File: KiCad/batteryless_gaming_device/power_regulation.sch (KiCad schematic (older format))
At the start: 16 parts, among them U500 TPS61201DRC

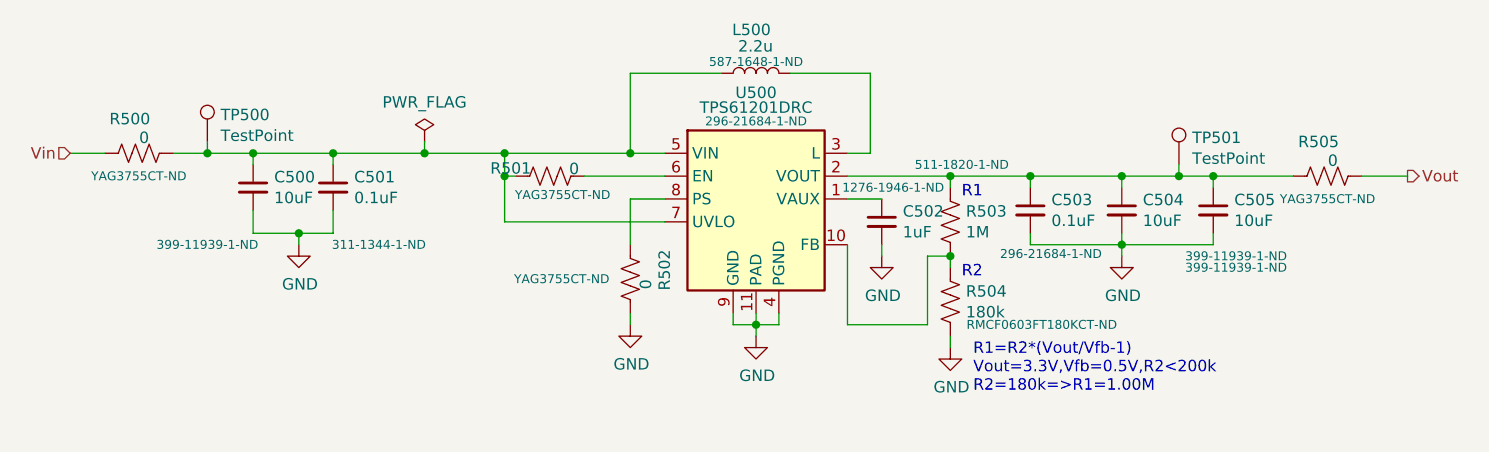
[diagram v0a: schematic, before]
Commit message: oh ya
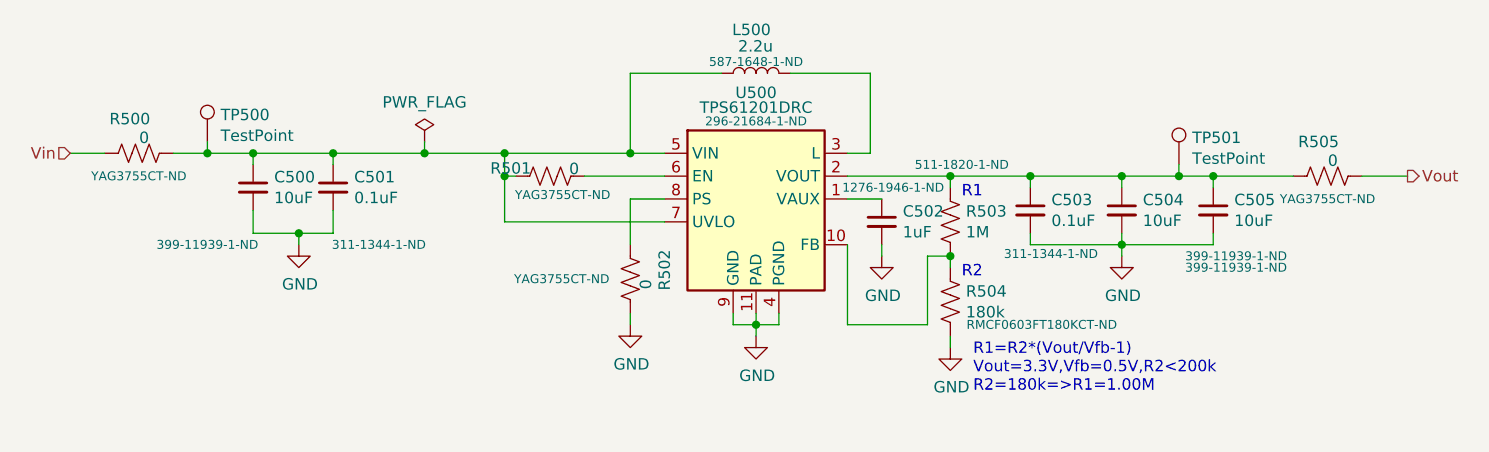
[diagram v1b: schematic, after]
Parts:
- C503: Digikey PN 296-21684-1-ND -> 311-1344-1-ND
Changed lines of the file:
@@
 F 2 "Capacitor_SMD:C_0603_1608Metric_Pad1.08x0.95mm_HandSolder" H 6500 4000 50  0001 C CNN
 F 3 "~" H 6500 4000 50  0001 C CNN
-F 4 "296-21684-1-ND" H 6590 3810 39  0000 C CNN "Digikey PN"
+F 4 "311-1344-1-ND" H 6590 3810 39  0000 C CNN "Digikey PN"
 	1    6500 4000
 	1    0    0    -1

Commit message: updated
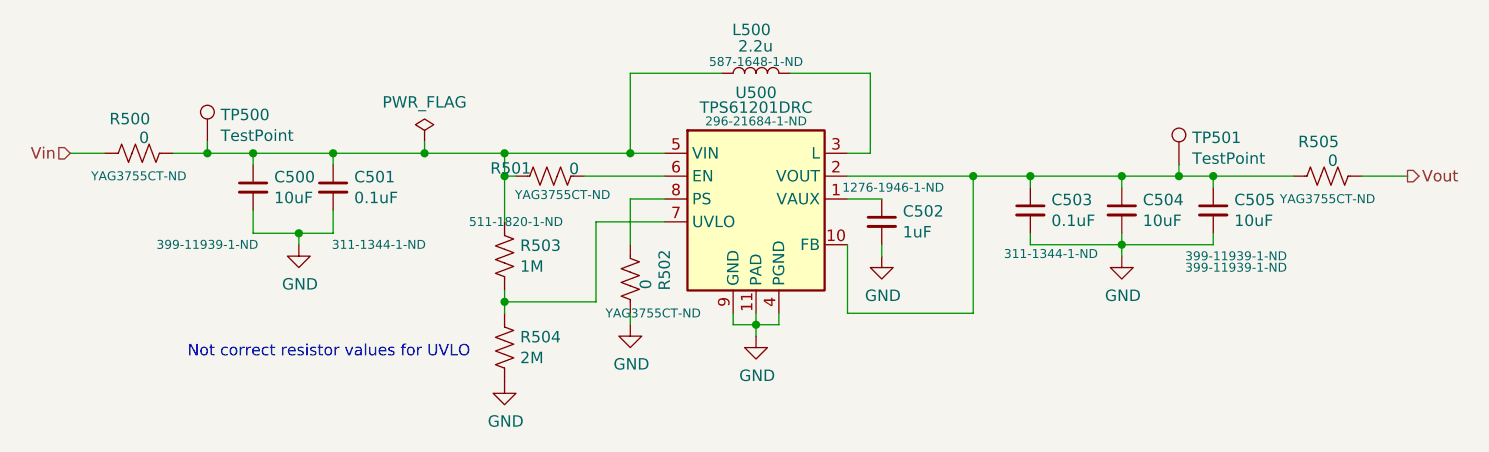
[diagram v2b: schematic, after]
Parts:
- R504: value 180k -> 2M; Digikey PN RMCF0603FT180KCT-ND -> (none)
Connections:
- net at R503.2, R504.1: now also U500.7 (UVLO); no longer U500.10 (FB)
- net at C503.1, C504.1, C505.1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: now also U500.10 (FB); no longer R503.1
- net at C500.1, C501.1, L500.1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: now also R503.1; no longer U500.7 (UVLO)
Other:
- note added: "Not correct resistor values for UVLO"
- note removed: "R1"
- note removed: "R1=R2*(Vout/Vfb-1)\nVout=3.3V,Vfb=0.5V,R2<200k\nR2=180k=>R1=1.00M"
- note removed: "R2"
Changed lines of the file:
@@
-	1    0    0    -1
-$EndComp
-$Comp
-L Device:R_US R?
-U 1 1 61950619
-P 6150 4050
-AR Path="/61950619" Ref="R?"  Part="1"
-AR Path="/61941831/61950619" Ref="R503"  Part="1"
-F 0 "R503" H 6218 4096 50  0000 L CNN
-F 1 "1M" H 6218 4005 50  0000 L CNN
-F 2 "Resistor_SMD:R_0603_1608Metric_Pad0.98x0.95mm_HandSolder" V 6190 4040 50  0001 C CNN
-F 3 "~" H 6150 4050 50  0001 C CNN
-F 4 "511-1820-1-ND" H 6200 4300 39  0000 C CNN "Digikey PN"
-	1    6150 4050
-	1    0    0    -1
-$EndComp
-$Comp
-L Device:R_US R?
-U 1 1 6195061F
-P 6150 4400
-AR Path="/6195061F" Ref="R?"  Part="1"
-AR Path="/61941831/6195061F" Ref="R504"  Part="1"
-F 0 "R504" H 6218 4446 50  0000 L CNN
-F 1 "180k" H 6218 4355 50  0000 L CNN
-F 2 "Resistor_SMD:R_0603_1608Metric_Pad0.98x0.95mm_HandSolder" V 6190 4390 50  0001 C CNN
-F 3 "~" H 6150 4400 50  0001 C CNN
-F 4 "RMCF0603FT180KCT-ND" H 6550 4300 39  0000 C CNN "Digikey PN"
-	1    6150 4400
 	1    0    0    -1
 $EndComp
@@
 	1    0    0    -1
 $EndComp
-Wire Wire Line
-	5700 3850 6150 3850
-Wire Wire Line
-	6150 3900 6150 3850
-Connection ~ 6150 3850
-Wire Wire Line
-	6150 3850 6500 3850
-Wire Wire Line
-	6150 4200 6150 4250
-$Comp
-L power:GND #PWR?
-U 1 1 61950666
-P 6150 4600
-AR Path="/61950666" Ref="#PWR?"  Part="1"
-AR Path="/61941831/61950666" Ref="#PWR0504"  Part="1"
-F 0 "#PWR0504" H 6150 4350 50  0001 C CNN
-F 1 "GND" H 6155 4427 50  0000 C CNN
-F 2 "" H 6150 4600 50  0001 C CNN
-F 3 "" H 6150 4600 50  0001 C CNN
-	1    6150 4600
-	1    0    0    -1
-$EndComp
-Wire Wire Line
-	6150 4600 6150 4550
-Wire Wire Line
-	6150 4200 6050 4200
-Wire Wire Line
-	6050 4200 6050 4500
-Wire Wire Line
-	6050 4500 5700 4500
-Wire Wire Line
-	5700 4500 5700 4150
-Connection ~ 6150 4200
-Text Notes 6250 4800 0    50   ~ 0
-R1=R2*(Vout/Vfb-1)\nVout=3.3V,Vfb=0.5V,R2<200k\nR2=180k=>R1=1.00M
-Text Notes 6200 3950 0    50   ~ 0
-R1
-Text Notes 6200 4300 0    50   ~ 0
-R2
 Wire Wire Line
 	2300 3750 2450 3750
@@
 F 2 "Resistor_SMD:R_0805_2012Metric_Pad1.20x1.40mm_HandSolder" V 4790 4290 50  0001 C CNN
 F 3 "~" H 4750 4300 50  0001 C CNN
-F 4 "YAG3755CT-ND" H 4450 4300 39  0000 C CNN "Digikey PN"
+F 4 "YAG3755CT-ND" H 4850 4150 39  0000 C CNN "Digikey PN"
 	1    4750 4300
 	1    0    0    -1
@@
 	4200 3850 4250 3850
 Wire Wire Line
-	4200 4050 4900 4050
-Wire Wire Line
 	4200 3850 4200 3750
 Connection ~ 4200 3850
@@
 Wire Wire Line
 	3850 3750 4200 3750
+$Comp
+L Device:R_US R?
+U 1 1 61B125C6
+P 4200 4200
+AR Path="/61B125C6" Ref="R?"  Part="1"
+AR Path="/61941831/61B125C6" Ref="R503"  Part="1"
+F 0 "R503" H 4268 4246 50  0000 L CNN
+F 1 "1M" H 4268 4155 50  0000 L CNN
+F 2 "Resistor_SMD:R_0603_1608Metric_Pad0.98x0.95mm_HandSolder" V 4240 4190 50  0001 C CNN
+F 3 "~" H 4200 4200 50  0001 C CNN
+F 4 "511-1820-1-ND" H 4250 4350 39  0000 C CNN "Digikey PN"
+	1    4200 4200
+	1    0    0    -1
+$EndComp
+Wire Wire Line
+	5700 3850 6250 3850
+$Comp
+L Device:R_US R?
+U 1 1 61B1718F
+P 4200 4600
+AR Path="/61B1718F" Ref="R?"  Part="1"
+AR Path="/61941831/61B1718F" Ref="R504"  Part="1"
+F 0 "R504" H 4268 4646 50  0000 L CNN
+F 1 "2M" H 4268 4555 50  0000 L CNN
+F 2 "Resistor_SMD:R_0603_1608Metric_Pad0.98x0.95mm_HandSolder" V 4240 4590 50  0001 C CNN
+F 3 "~" H 4200 4600 50  0001 C CNN
+F 4 "" H 3950 4750 39  0000 C CNN "Digikey PN"
+	1    4200 4600
+	1    0    0    -1
+$EndComp
+$Comp
+L power:GND #PWR?
+U 1 1 61B17DBB
+P 4200 4750
+AR Path="/61B17DBB" Ref="#PWR?"  Part="1"
+AR Path="/61941831/61B17DBB" Ref="#PWR0115"  Part="1"
+F 0 "#PWR0115" H 4200 4500 50  0001 C CNN
+F 1 "GND" H 4205 4577 50  0000 C CNN
+F 2 "" H 4200 4750 50  0001 C CNN
+F 3 "" H 4200 4750 50  0001 C CNN
+	1    4200 4750
+	1    0    0    -1
+$EndComp
+Wire Wire Line
+	4200 4450 4200 4400
+Wire Wire Line
+	4200 4400 4600 4400
+Wire Wire Line
+	4600 4400 4600 4050
+Wire Wire Line
+	4600 4050 4900 4050
+Connection ~ 4200 4400
+Wire Wire Line
+	4200 4400 4200 4350
+Wire Wire Line
+	5700 4150 5700 4450
+Wire Wire Line
+	5700 4450 6250 4450
+Wire Wire Line
+	6250 4450 6250 3850
+Connection ~ 6250 3850
+Wire Wire Line
+	6250 3850 6500 3850
+Text Notes 4050 4650 2    50   ~ 0
+Not correct resistor values for UVLO
 $EndSCHEMATC
